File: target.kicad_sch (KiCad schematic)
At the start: 18 parts, among them J2 3020-10-0100-00, Q1 DMG1012UW-7, Q2 DMG1012UW-7, U5 FXLA108BQX, U6 AP22804AW5-7

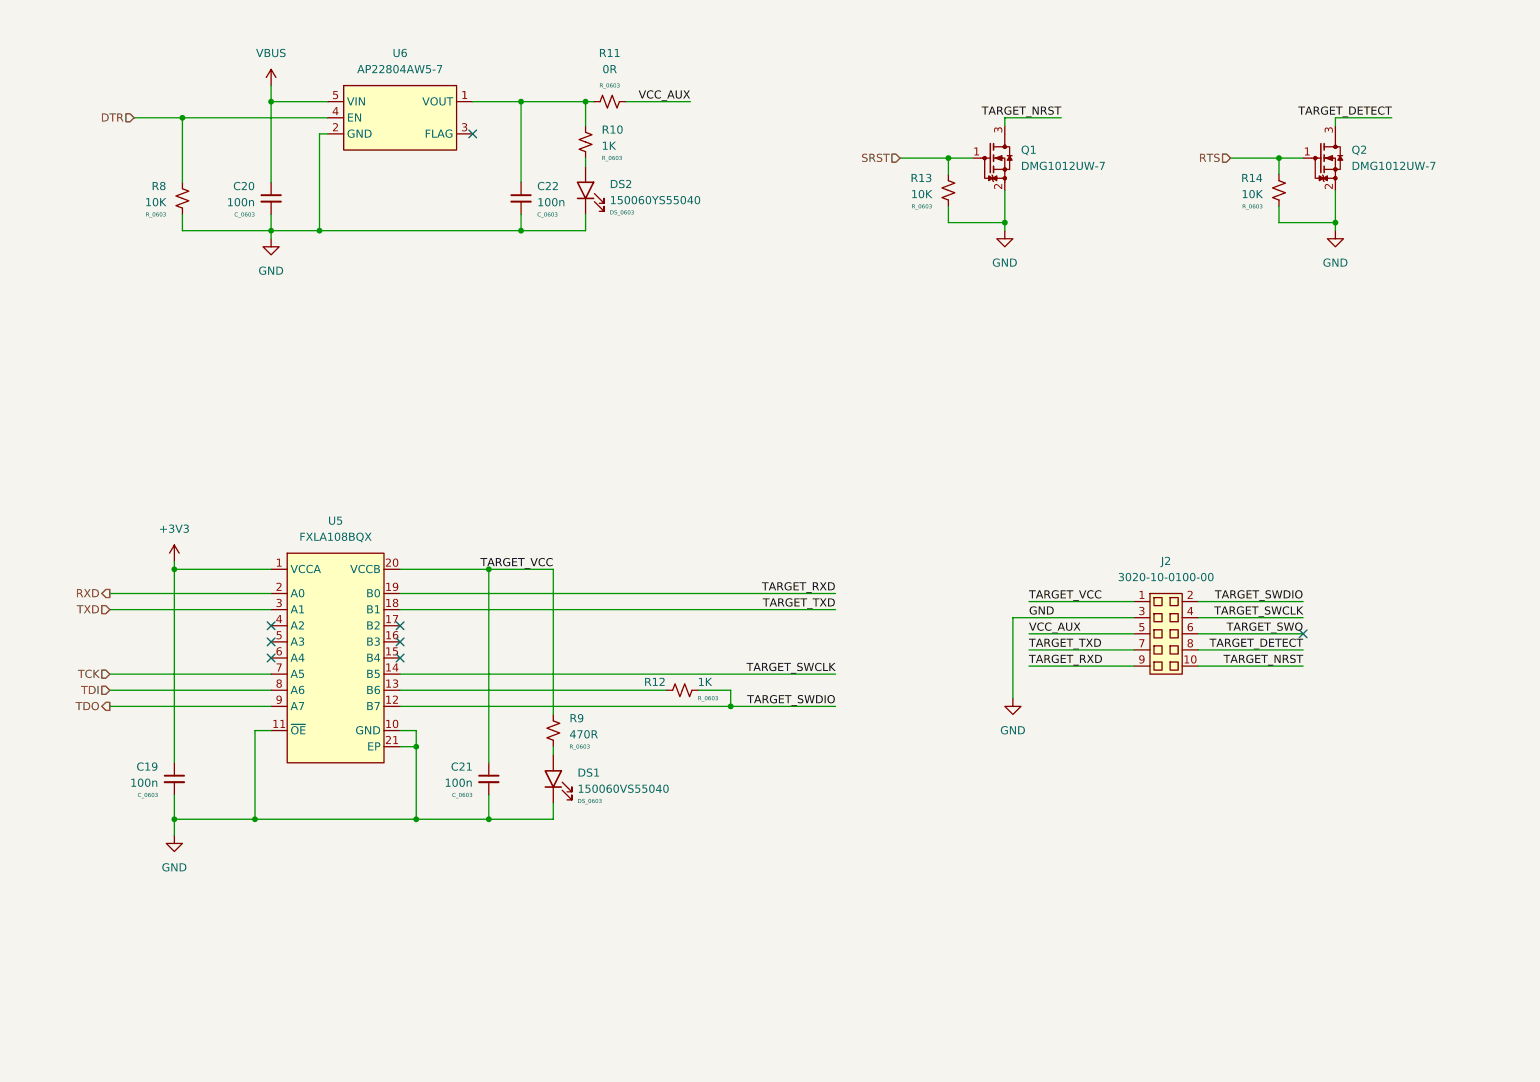
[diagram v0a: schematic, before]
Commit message: Rework logic gates
Rename to aphid
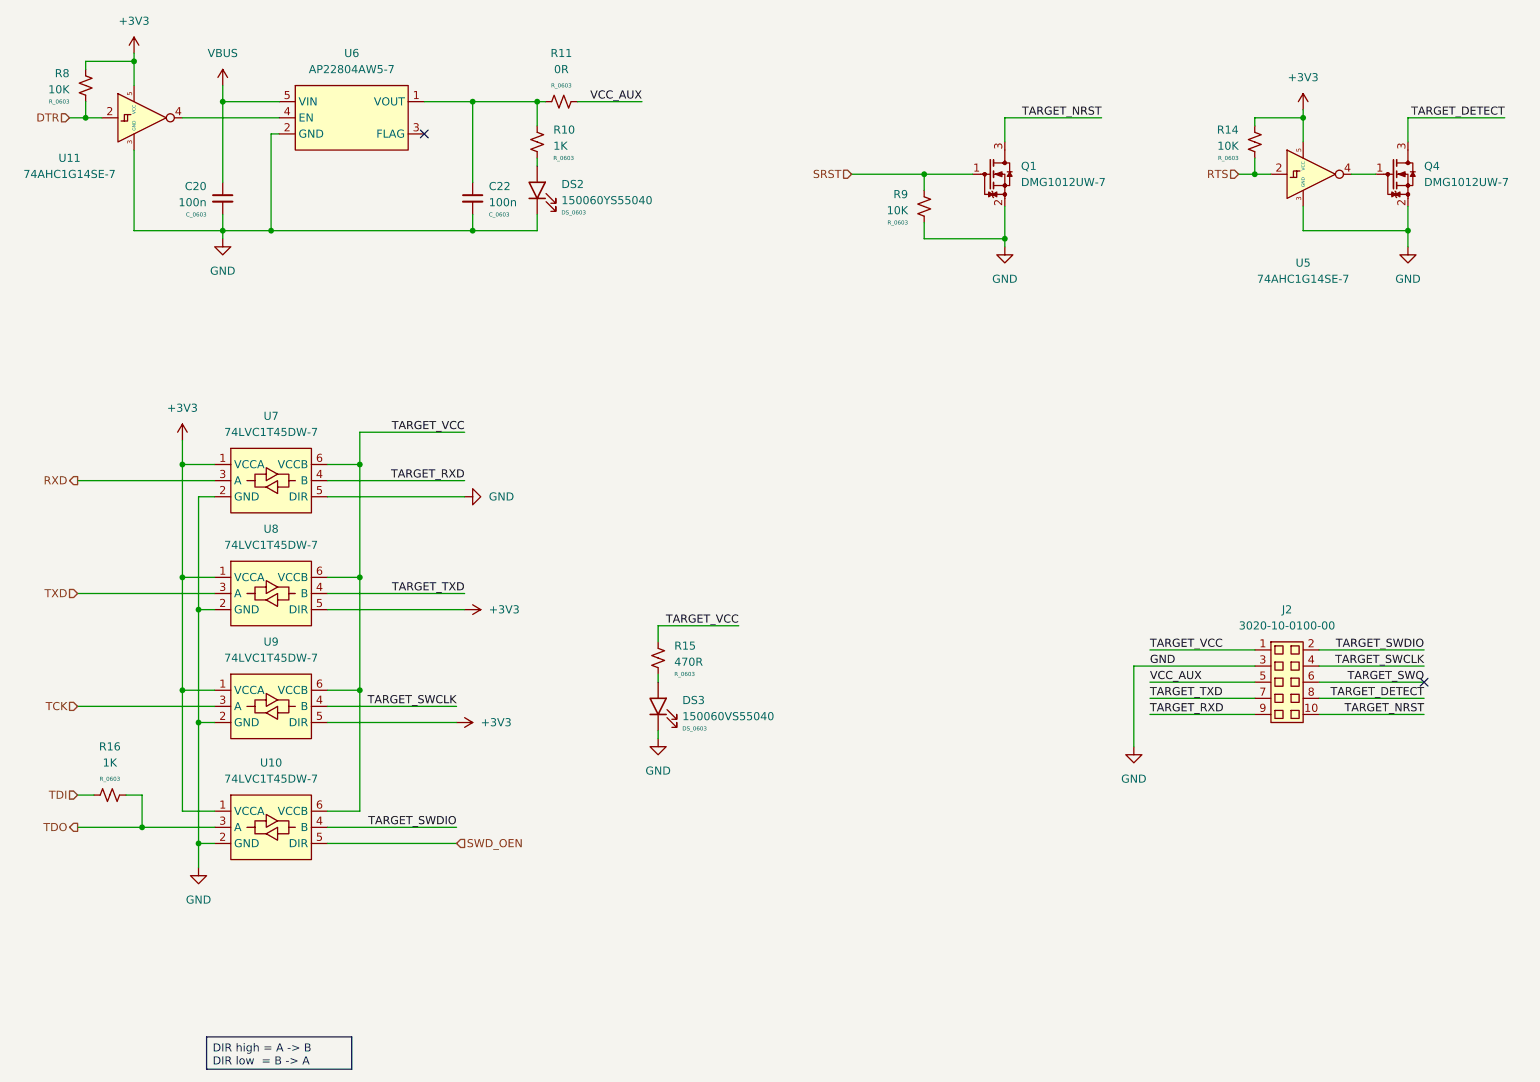
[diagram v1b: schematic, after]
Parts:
- removed C19, C21: 100n, C_Capacitor:C_0603, symbol C_Capacitor:C_0603
- removed DS1: 150060VS55040, DS_LED:DS_0603, symbol DS_LED:150060VS55040
- removed Q2: DMG1012UW-7, U_IC:SC70-3, symbol Q_MOSFET:DMG1012UW-7
- removed R12: 1K, R_Resistor:R_0603, symbol R_Resistor:R_0603
- removed R13: 10K, R_Resistor:R_0603, symbol R_Resistor:R_0603
- removed U5: FXLA108BQX, U_IC:WQFN20_05_4.5x2.5, symbol U_Basic:FXLA108BQX
- added DS3: 150060VS55040, DS_LED:DS_0603, symbol DS_LED:150060VS55040
- added Q4: DMG1012UW-7, U_IC:SC70-3, symbol Q_MOSFET:DMG1012UW-7
- added R15: 470R, R_Resistor:R_0603, symbol R_Resistor:R_0603
- added R16: 1K, R_Resistor:R_0603, symbol R_Resistor:R_0603
- added U10, U7, U8, U9: 74LVC1T45DW-7, U_IC:SC70-6, symbol U_Logic:74LVC1T45DW-7
- added U11, U5: 74AHC1G14SE-7, U_IC:SC70-5, symbol U_Logic:74AHC1G14SE-7
- R9: value 470R -> 10K
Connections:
- net +3V3: now also R14.1, R8.1, U10.1 (VCCA), U11.5 (VCC), U5.5 (VCC), U7.1 (VCCA), U8.1 (VCCA), U8.5 (DIR), U9.1 (VCCA), U9.5 (DIR)
- net DTR: now also R8.2, U11.2; no longer R8.1, U6.4 (EN)
- net GND: now also R9.2, DS3.1 (K), Q4.2 (S), U10.2 (GND), U11.3 (GND), U5.3 (GND), U7.2 (GND), U7.5 (DIR), U8.2 (GND), U9.2 (GND); no longer R14.2, R8.2
- net RTS: now also R14.2, U5.2; no longer R14.1
- net RXD: now also U7.3 (A)
- net SRST: now also R9.1
- net TARGET_DETECT: now also Q4.3 (D)
- net TARGET_RXD: now also U7.4 (B)
- net TARGET_SWCLK: now also U9.4 (B)
- net TARGET_SWDIO: now also U10.4 (B)
- net TARGET_TXD: now also U8.4 (B)
- net TARGET_VCC: now also R15.1, U10.6 (VCCB), U7.6 (VCCB), U8.6 (VCCB), U9.6 (VCCB); no longer R9.1
- net TCK: now also U9.3 (A)
- net TDI: now also R16.1
- net TDO: now also R16.2, U10.3 (A)
- net TXD: now also U8.3 (A)
- new net: U11.4, U6.4 (EN)
- new net: DS3.2 (A), R15.2
- new net: Q4.1 (G), U5.4
- new net SWD_OEN: U10.5 (DIR)
- no-connect marks 8 -> 2
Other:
- title: X-Link -> Aphid
- moved on the sheet: C20, C22, DS2, J2, R10, R11, U6
